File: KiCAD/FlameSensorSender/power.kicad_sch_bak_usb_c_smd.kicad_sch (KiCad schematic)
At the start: 26 parts, among them J5 Conn_01x06_Socket, J6 Conn_01x06_Pin, J7 6 Pin USB-C Type USB Connecto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, Q3 AO3400A, U3 TPS63802DLAR, U4 TPS63802DLAR

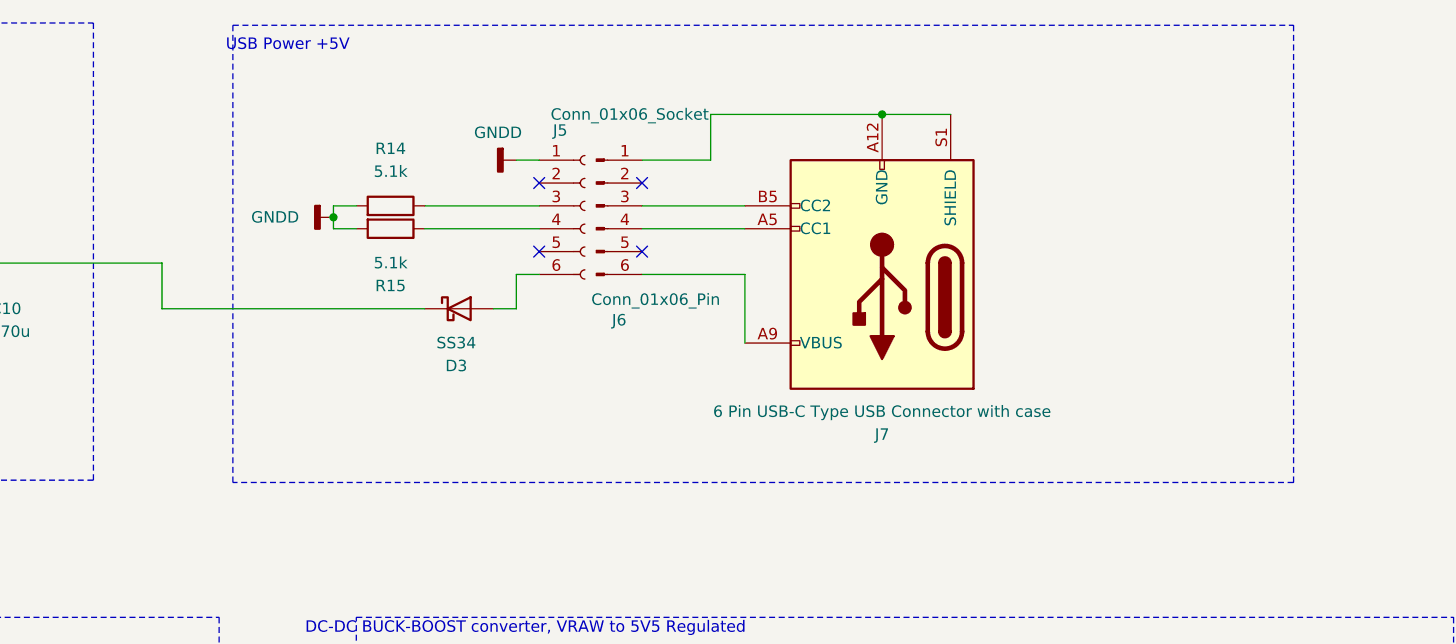
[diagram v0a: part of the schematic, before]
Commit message: dev
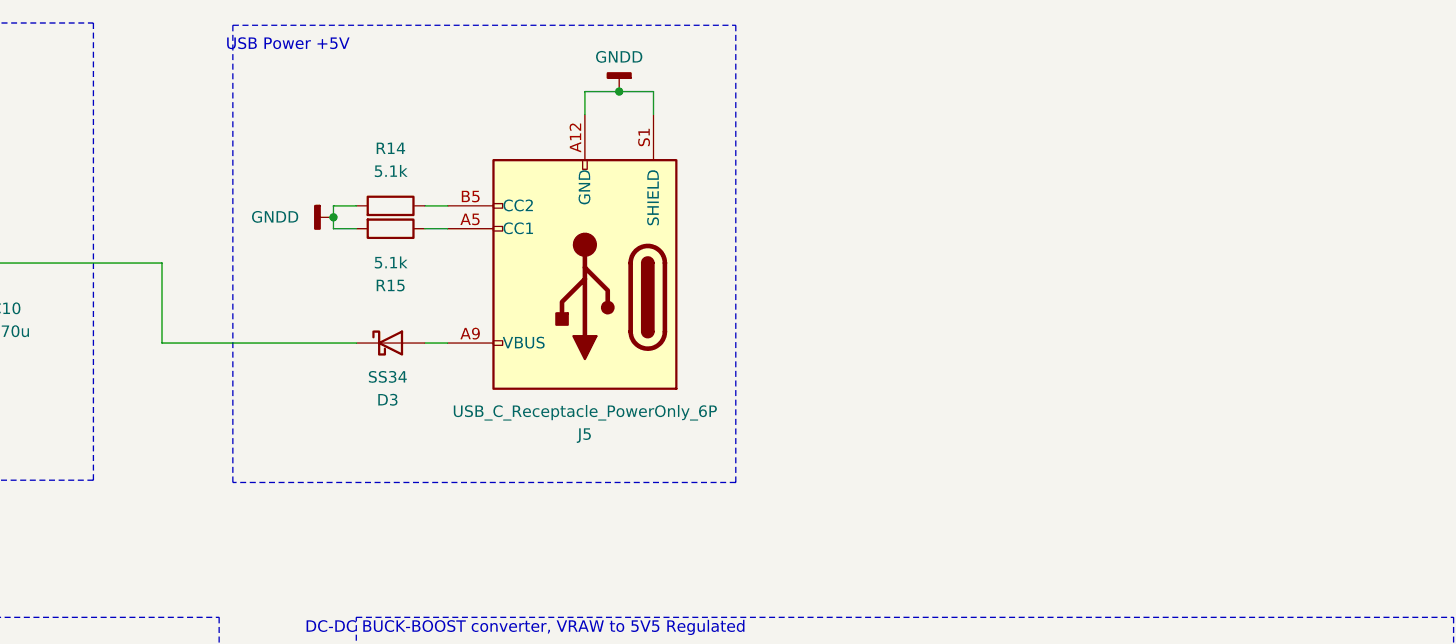
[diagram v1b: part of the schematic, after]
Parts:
- removed J5: Conn_01x06_Socket, Connector_JST:JST_PH_S6B-PH-K_1x06_P2.00mm_Horizontal, symbol Connector:Conn_01x06_Socket
- removed J6: Conn_01x06_Pin, symbol Connector:Conn_01x06_Pin
- J5: renamed from J7; value 6 Pin USB-C Type USB Connector with case -> USB_C_Receptacle_PowerOnly_6P; footprint (none) -> Connector_USB:USB_C_Receptacle_GCT_USB4135-GF-A_6P_TopMnt_Horizontal
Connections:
- net GNDD: now also J5.A12 (GND), J5.B12 (GND), J5.S1 (SHIELD)
- net at R14.1: now also J5.B5 (CC2)
- net at R15.1: now also J5.A5 (CC1)
- net at D3.2 (A): now also J5.A9 (VBUS), J5.B9 (VBUS)
- no-connect marks 4 -> 0
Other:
- moved on the sheet: D3, J5
